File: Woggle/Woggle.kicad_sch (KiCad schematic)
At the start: 23 parts, among them SW1 SW_SPDT, SW2 Sequance, U1 ATtiny85-20P

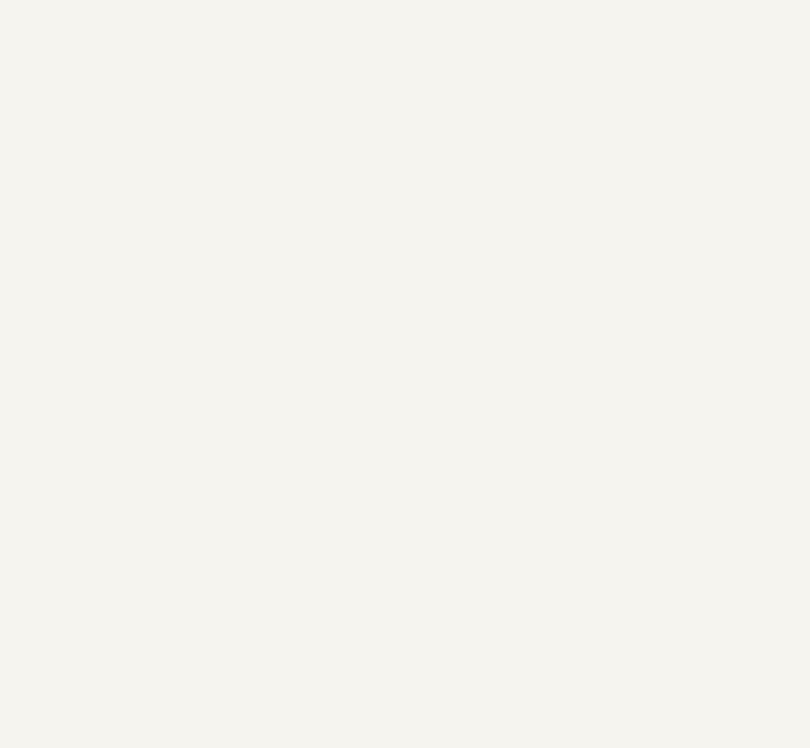
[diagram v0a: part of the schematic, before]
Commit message: .
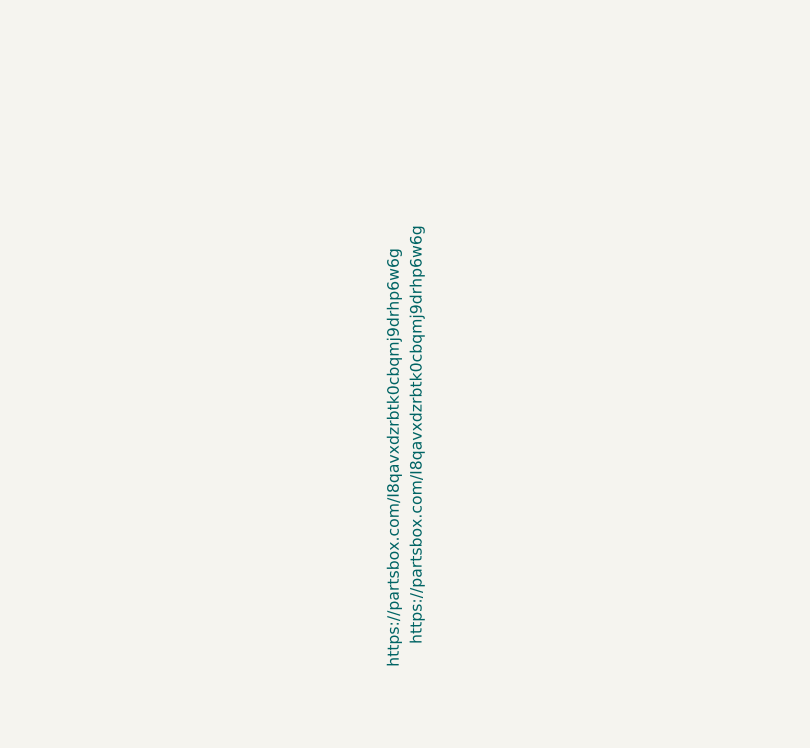
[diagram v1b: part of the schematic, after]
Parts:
- R1, R2, R3, R4: Partsbox (none) -> https://partsbox.com/I8qavxdzrbtk0cbqmj9drhp6w6g
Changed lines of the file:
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@@
+			)
+		)
+		(property "Partsbox" "https://partsbox.com/I8qavxdzrbtk0cbqmj9drhp6w6g"
+			(at 123.19 229.87 0)
+			(show_name no)
+			(do_not_autoplace no)
+			(effects
+				(font
+					(size 1.27 1.27)
+				)
 			)
 		)
@@
 			)
 		)
+		(property "Partsbox" "https://partsbox.com/I8qavxdzrbtk0cbqmj9drhp6w6g"
+			(at 176.53 58.42 90)
+			(hide yes)
+			(show_name no)
+			(do_not_autoplace no)
+			(effects
+				(font
+					(size 1.27 1.27)
+				)
+			)
+		)
 		(pin "1"
 		)
@@
 			)
 		)
+		(property "Partsbox" "https://partsbox.com/I8qavxdzrbtk0cbqmj9drhp6w6g"
+			(at 176.53 60.96 90)
+			(hide yes)
+			(show_name no)
+			(do_not_autoplace no)
+			(effects
+				(font
+					(size 1.27 1.27)
+				)
+			)
+		)
 		(pin "1"
 		)
@@
 			(show_name no)
 			(do_not_autoplace no)
+			(effects
+				(font
+					(size 1.27 1.27)
+				)
+			)
+		)
+		(property "Partsbox" "https://partsbox.com/I8qavxdzrbtk0cbqmj9drhp6w6g"
+			(at 120.65 232.41 0)
+			(show_name no)
+			(do_not_autoplace no)
